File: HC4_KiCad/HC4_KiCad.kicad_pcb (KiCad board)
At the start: 2 copper layers, 150 x 150 mm, 155 parts, among them IC1 RAM, IC10 74HC4002, IC11 74HC161, IC12 74HC377, IC13 74HC161, IC14 74HC161, IC15 74HC161, IC16 74HC257, IC17 74HC257, IC18 74HC00, IC19 74HC32, IC2 ROM, IC20 74HC74, IC21 74HC4053, IC22 74HC04, IC23 74HC151, IC24 74HC14, IC3 74HC153, IC4 74HC153, IC5 74HC153, IC6 74HC153, IC7 74HC283, IC8 74HC244, IC8 74HC257, IC9 74HC244, J1 Power, J2 CE, J3 Expantion_Connector, SW1 SW_SPDT, SW2 Bus_Open, SW3 SW_Push, SW4 SW_Push, SW5 SW_SPDT

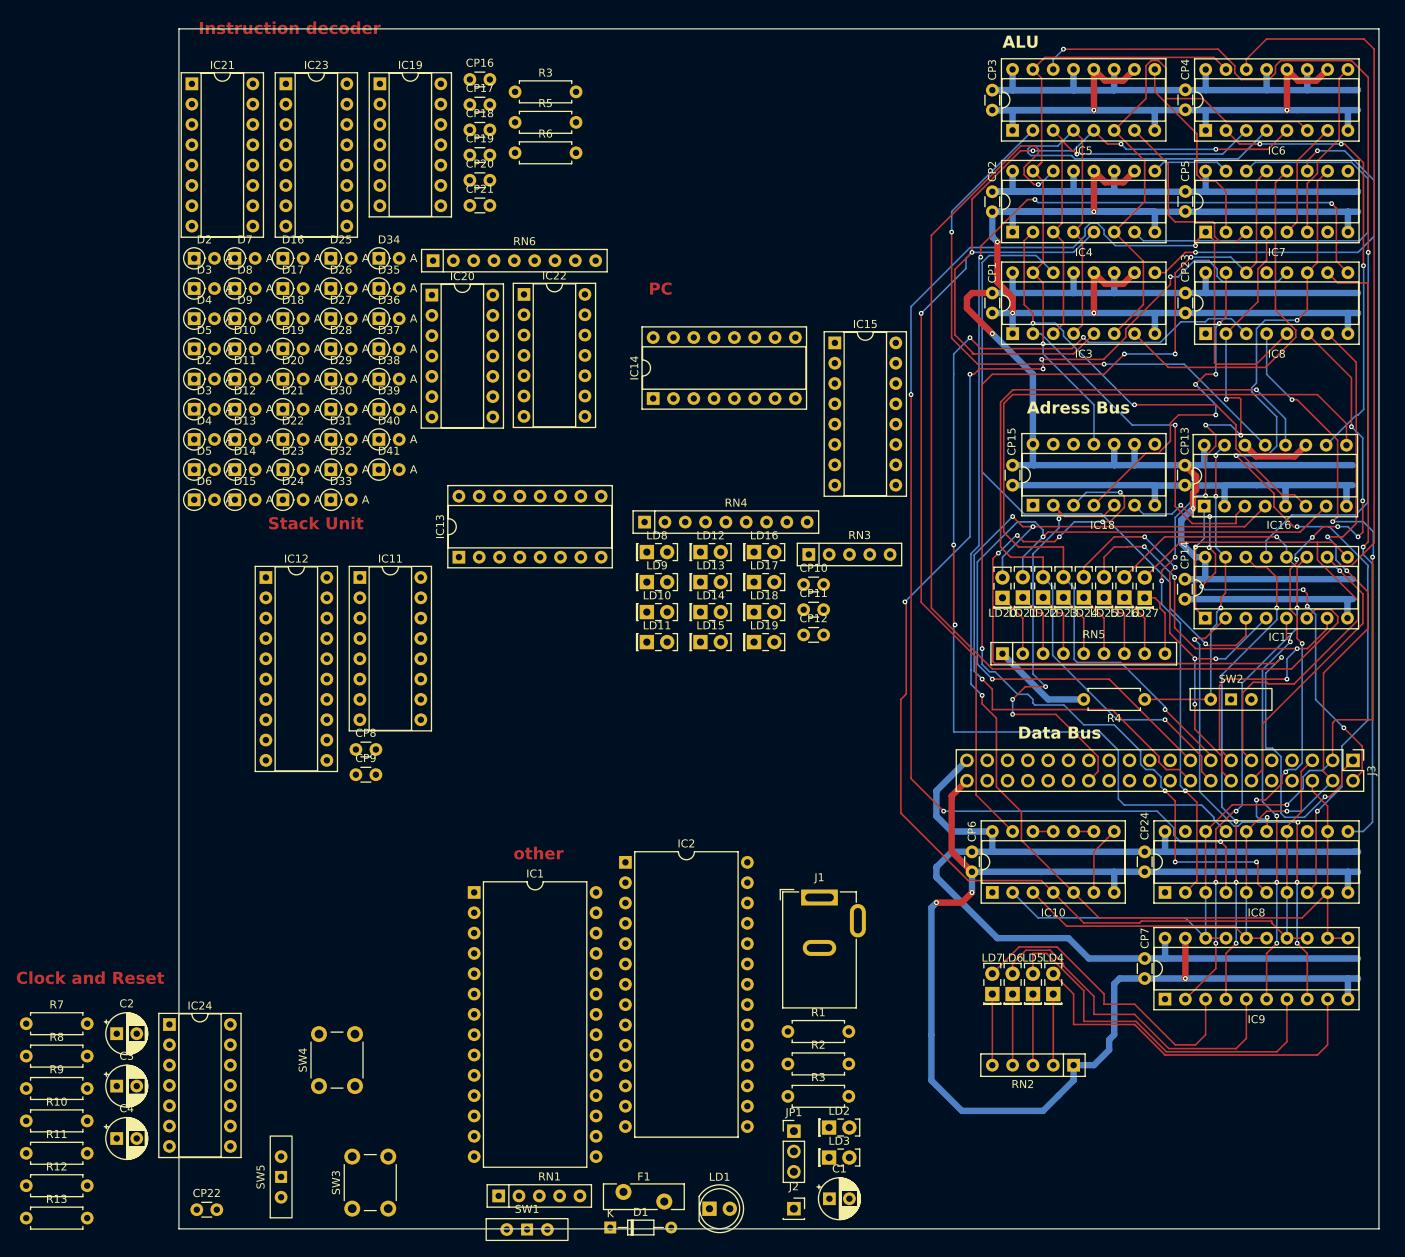
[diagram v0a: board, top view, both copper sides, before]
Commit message: 更地になった。
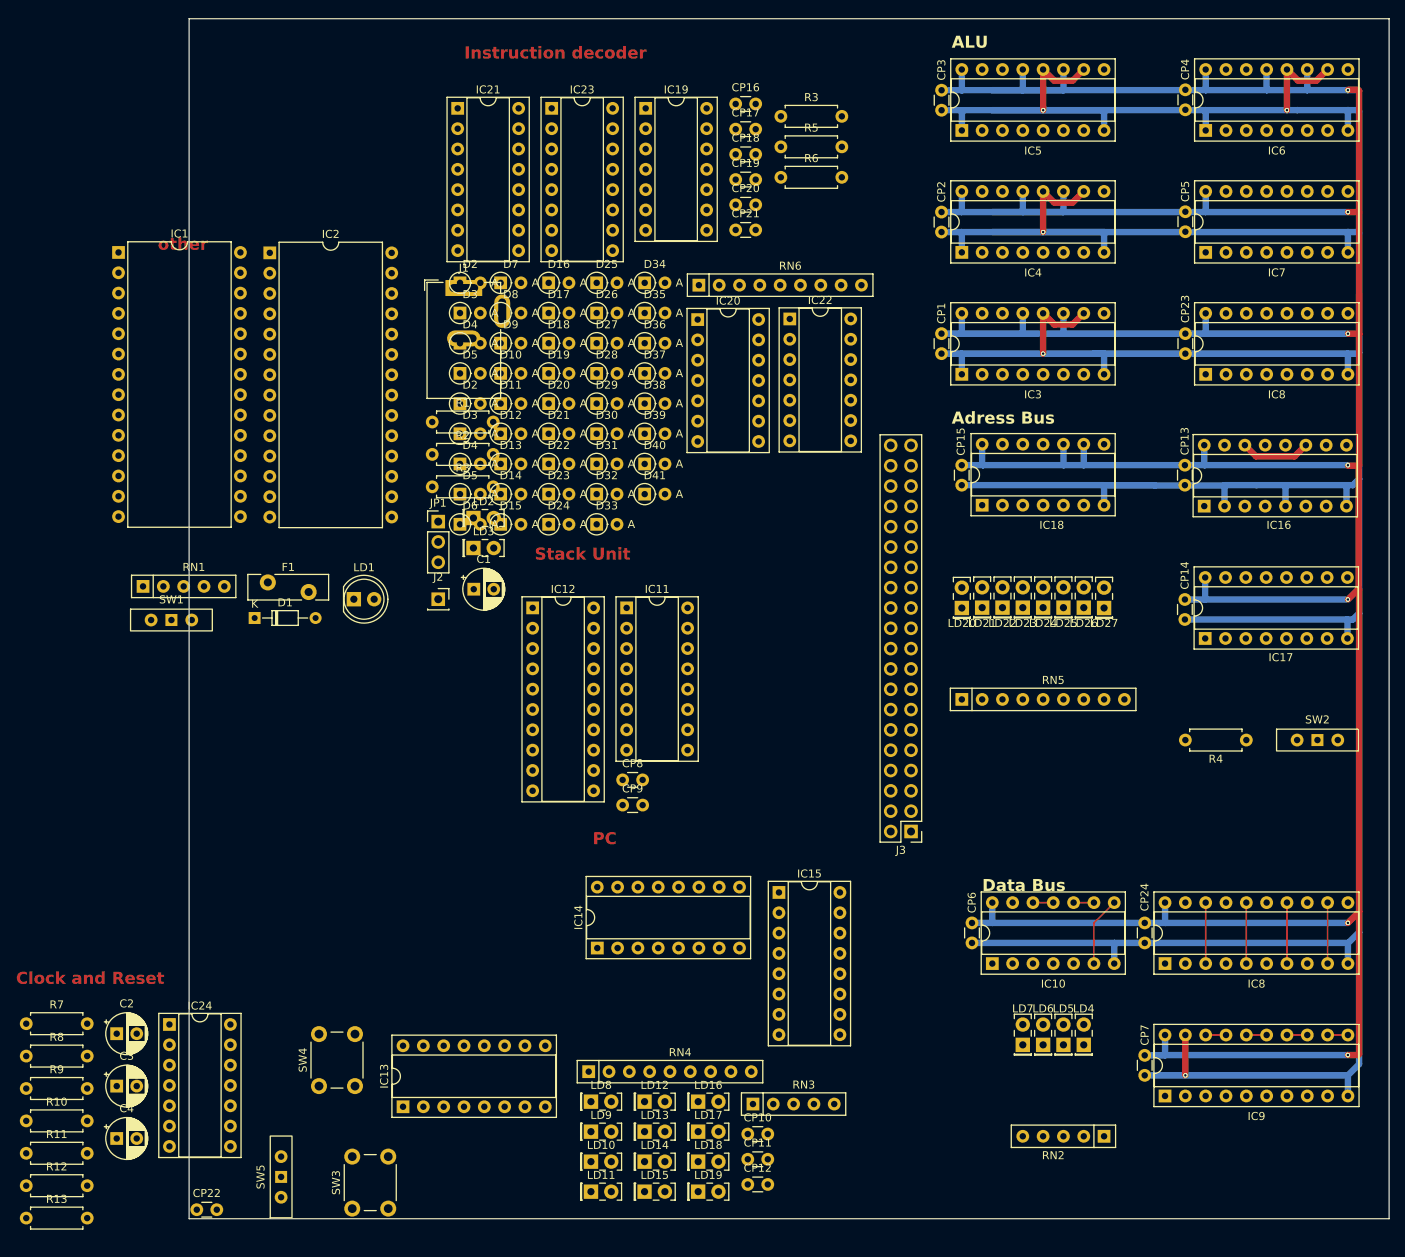
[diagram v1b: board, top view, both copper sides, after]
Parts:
- moved IC1 91.5 mm to (82.5, 53.4)
- moved D1 88.2 mm to (99.6, 99.0)
- moved J1 88.2 mm to (125.7, 57.8)
- moved LD2 88.2 mm to (126.9, 86.5)
- moved LD3 88.2 mm to (126.9, 90.3)
- moved R1 88.2 mm to (121.8, 74.5)
- moved R3 88.2 mm to (121.8, 82.6)
- moved SW1 88.2 mm to (89.2, 99.3)
- moved C1 88.2 mm to (126.9, 95.4)
- moved F1 88.2 mm to (101.2, 94.6)
- moved IC2 88.2 mm to (101.5, 53.4)
- moved J2 88.2 mm to (122.5, 96.7)
- moved JP1 88.2 mm to (122.5, 87.0)
- moved LD1 88.2 mm to (112.0, 96.7)
- moved R2 88.2 mm to (121.8, 78.6)
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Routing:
- net /Data BUS/Stack3: track 200.0 -> 10.2 mm, vias 4 -> 0
- net /ALU/ALU_OUT1: track 179.8 -> 0.00 mm, vias 4 -> 0
- net /Data BUS/Stack2: track 189.4 -> 10.2 mm, vias 5 -> 0
- net /ALU/I1a: track 179.0 -> 0.57 mm, vias 5 -> 0
- net /ALU/ALU_OUT2: track 150.4 -> 0.00 mm, vias 7 -> 0
- net /ALU/ALU_in_A2: track 135.3 -> 0.00 mm, vias 1 -> 0
- net /Data BUS/Level_C0: track 131.1 -> 0.00 mm, vias 4 -> 0
- net /Data BUS/Stack0: track 129.7 -> 10.2 mm, vias 4 -> 0
- net /ALU/ALU_in_A1: track 115.6 -> 0.00 mm, vias 2 -> 0
- net /ALU/ALU_OUT3: track 114.8 -> 0.00 mm, vias 4 -> 0
- net /Data BUS/Stack1: track 123.1 -> 10.2 mm, vias 3 -> 0
- net /Address BUS/~{RAM_RD}: track 112.4 -> 0.00 mm, vias 7 -> 0
- net /Address BUS/RAM_A4: track 109.3 -> 0.00 mm, vias 1 -> 0
- net /Address BUS/RAM_A5: track 105.1 -> 0.00 mm, vias 2 -> 0
- net /Address BUS/RAM_A6: track 99.3 -> 0.00 mm, vias 2 -> 0
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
